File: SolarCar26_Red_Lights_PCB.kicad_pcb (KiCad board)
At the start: 2 copper layers, 79 x 11 mm, 9 parts, among them J1 Conn_01x02

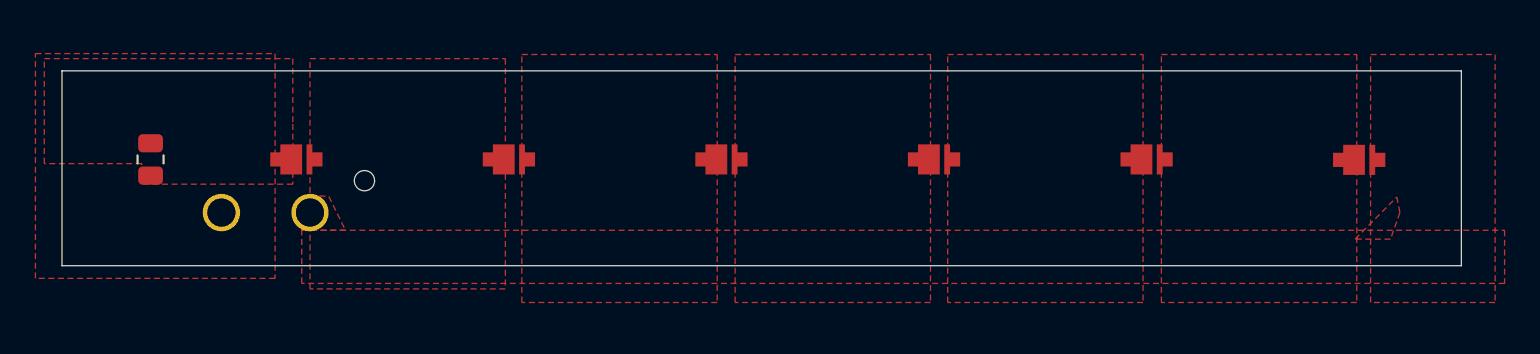
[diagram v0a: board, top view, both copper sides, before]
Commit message: Add files via upload
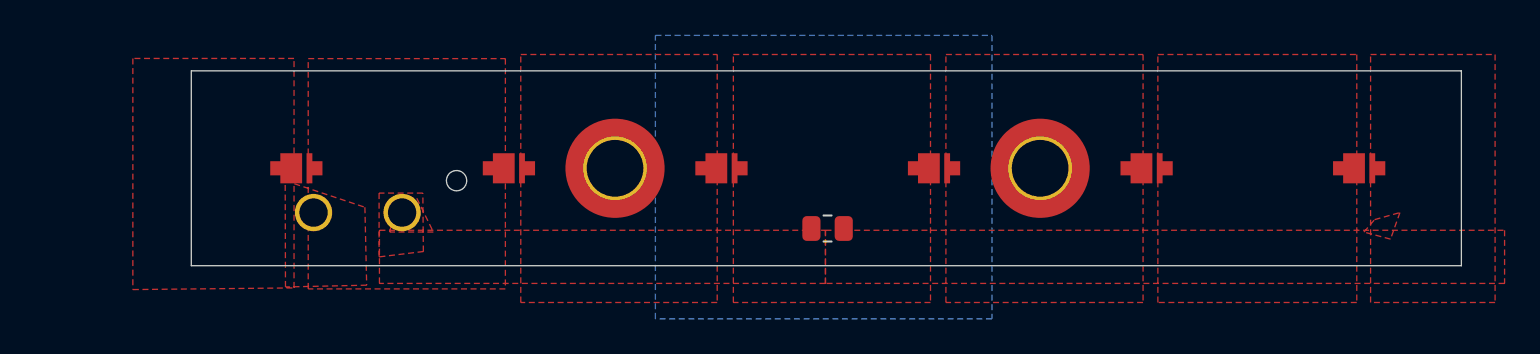
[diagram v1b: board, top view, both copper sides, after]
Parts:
- added REF**: MountingHole_3.2mm_M3_DIN965_Pad_TopOnly, MountingHole:MountingHole_3.2mm_M3_DIN965_Pad_TopOnly, F.Cu at (72.2, 91.5)
- added REF**: MountingHole_3.2mm_M3_DIN965_Pad_TopOnly, MountingHole:MountingHole_3.2mm_M3_DIN965_Pad_TopOnly, F.Cu at (96.2, 91.5)
- moved R1 38.4 mm to (84.2, 94.9), turned to 0 degrees
- moved J1 5.20 mm to (55.2, 94.0)
- moved D1 0.50 mm to (55.0, 91.5)
- moved D2 0.50 mm to (67.0, 91.5)
- moved D3 0.50 mm to (79.0, 91.5)
- moved D4 0.50 mm to (91.0, 91.5)
- moved D5 0.50 mm to (103.0, 91.5)
- moved D6 0.47 mm to (115.0, 91.5)
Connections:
- D1 pad 2: Net-(D1-A) -> /+12V
- J1 pad 1: Net-(J1-Pin_1) -> /+12V
- J1 pad 2: Net-(D6-K) -> /GND
- R1 pad 1: Net-(J1-Pin_1) -> /GND
- R1 pad 2: Net-(D1-A) -> Net-(D6-K)
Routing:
- added copper zone on B.Cu, net (none)
- added copper zone on F.Cu, net /+12V
- added copper zone on F.Cu, net /GND
- removed copper zone on F.Cu, net Net-(D1-A)
- removed copper zone on F.Cu, net Net-(J1-Pin_1)
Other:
- board size 79 x 11 mm -> 71.7 x 11 mm
- board text added: "BSEE VT 2028"
- board text added: "Savannah Exley"
- board text removed: "Savannah Exley Electrical Engineering VT 2028"
